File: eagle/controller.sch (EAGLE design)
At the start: 11 parts, among them K1 SRD-05VDC-SL-C, K2 SRD-05VDC-SL-C, K3 SRD-05VDC-SL-C, K4 SRD-05VDC-SL-C

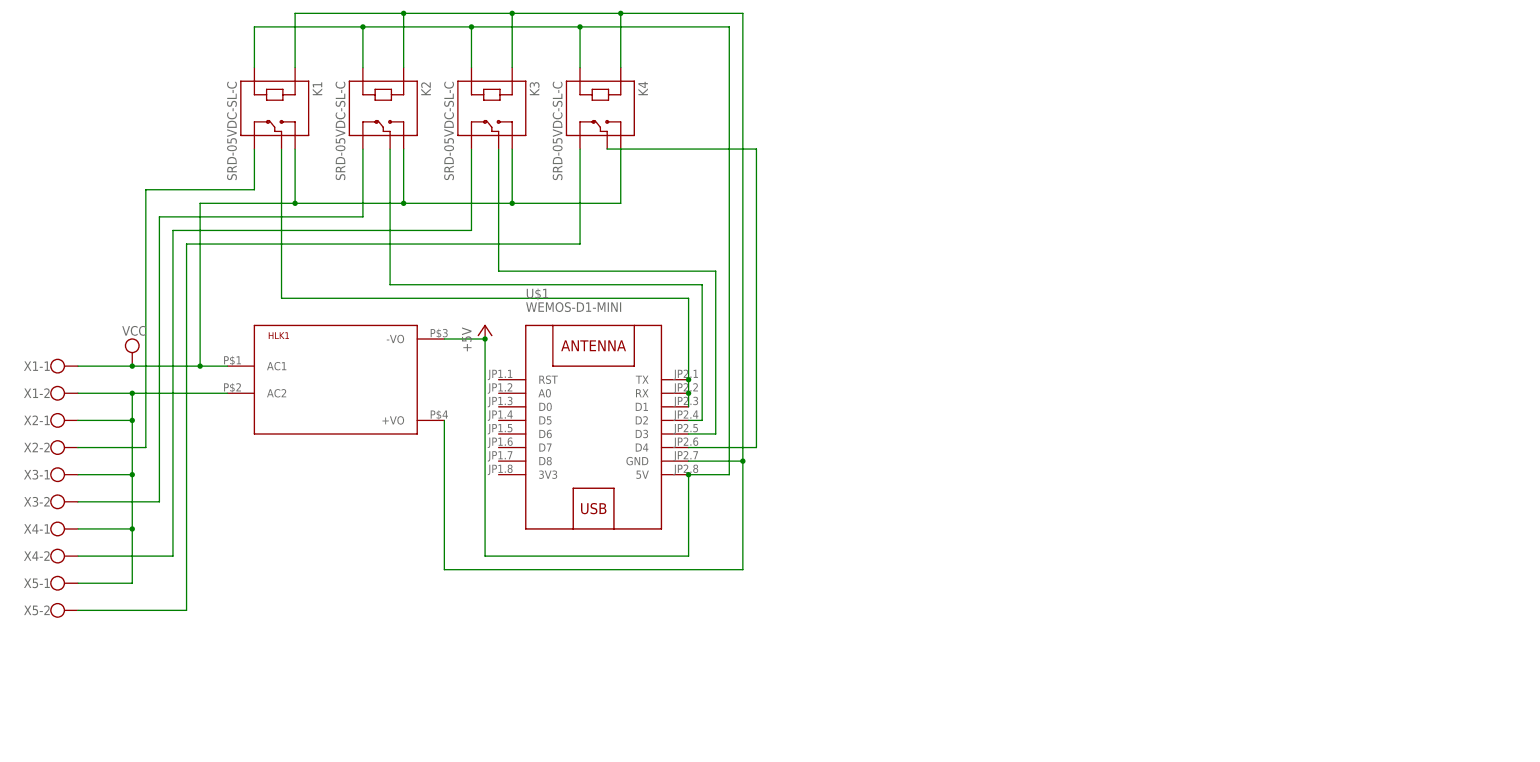
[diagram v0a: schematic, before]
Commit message: WIP
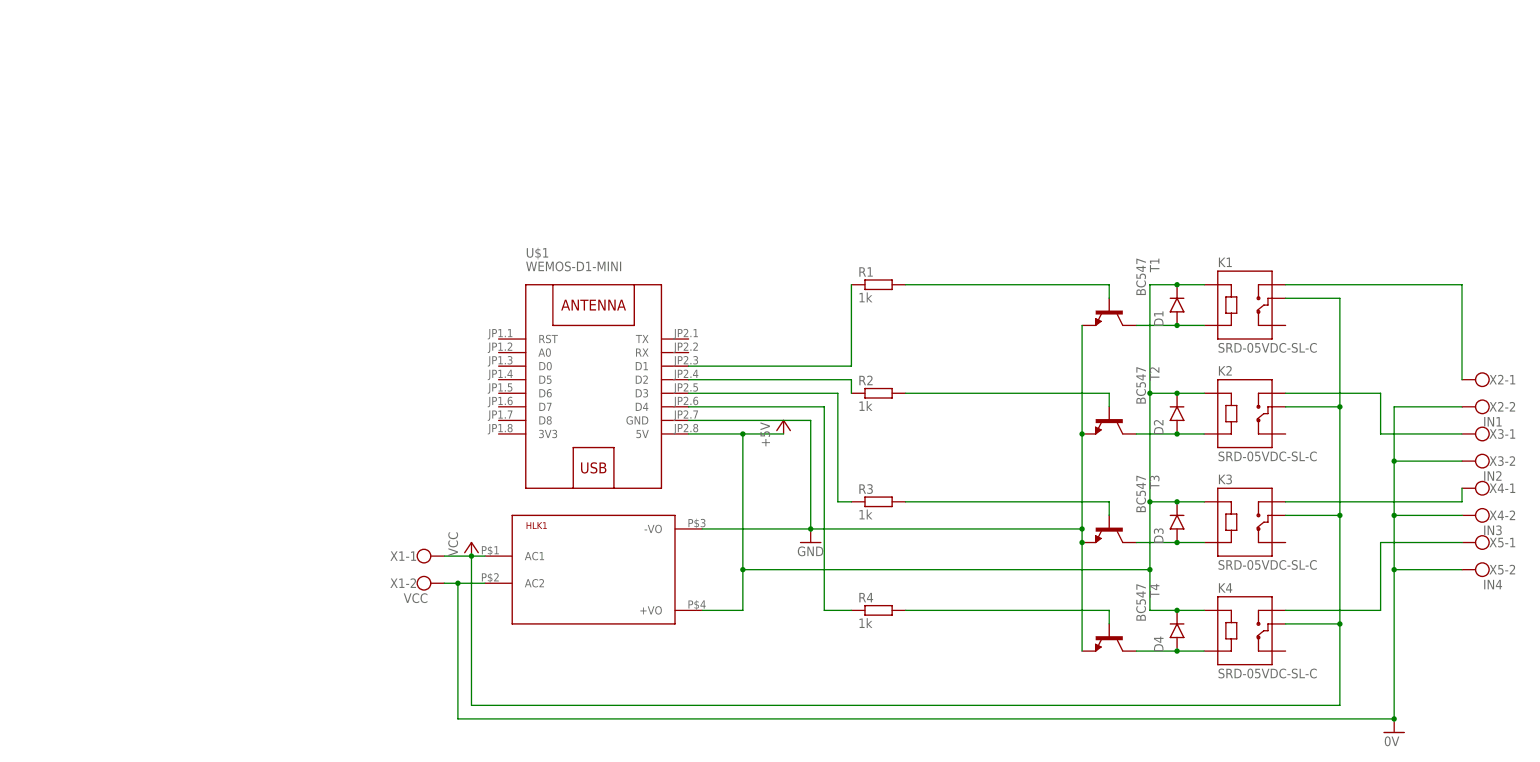
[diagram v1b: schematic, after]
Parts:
- added D1, D2, D3, D4: 1N4001, tango:1N4001
- added R1, R2, R3, R4: 1k, rcl:R-EU_0204/5
- added T1, T2, T3, T4: BC547, transistor:BC547
- X1: value (none) -> VCC
- X2: value (none) -> IN1
- X3: value (none) -> IN2
- X4: value (none) -> IN3
- X5: value (none) -> IN4
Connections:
- removed net N$6: K2.NC, X3-2.KL
- new net 0V: HLK1.AC2, X1-2.KL, X2-2.KL, X3-2.KL, X4-2.KL, X5-2.KL
- new net GND: HLK1.-VO, T1.E, T2.E, T3.E, T4.E, U$1.GND
- new net N$1: D1.ANODE, K1.A2, T1.C
- new net N$10: R4.2, T4.B
- new net N$13: K4.NO, X5-1.KL
- new net N$14: R1.1, U$1.D1
- new net N$15: R2.1, U$1.D2
- new net N$16: R3.1, U$1.D3
- new net N$17: R4.1, U$1.D4
- net +5V: now also D1.CATHODE, D2.CATHODE, D3.CATHODE, D4.CATHODE, HLK1.+VO, K1.A1, K2.A1, K3.A1, K4.A1; no longer HLK1.-VO, K1.A2, K2.A2, K3.A2, K4.A2
- net N$11: now also K2.NO, X3-1.KL; no longer HLK1.+VO, K1.A1, K2.A1, K3.A1, K4.A1, U$1.GND
- net N$12: now also K3.NO; no longer HLK1.AC2, X1-2.KL, X2-1.KL, X3-1.KL, X5-1.KL
- net N$2: now also K1.NO, X2-1.KL; no longer K1.COM, U$1.D1, U$1.RX, U$1.TX
- net N$3: now also D2.ANODE, K2.A2, T2.C; no longer K2.COM, U$1.D2
- net N$4: now also D3.ANODE, K3.A2, T3.C; no longer K4.NC, X5-2.KL
- net N$5: now also D4.ANODE, K4.A2, T4.C; no longer K3.NC, X4-2.KL
- net N$7: now also R3.2, T3.B; no longer K1.NC, X2-2.KL
- net N$8: now also R2.2, T2.B; no longer K3.COM, U$1.D3
- net N$9: now also R1.2, T1.B; no longer K4.COM, U$1.D4
- net VCC: now also K1.COM, K2.COM, K3.COM, K4.COM; no longer K1.NO, K2.NO, K3.NO, K4.NO
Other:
- moved on the sheet: HLK1, K1, K2, K3, K4, U$1, X1-1, X1-2, X2-1, X2-2, X3-1, X3-2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
